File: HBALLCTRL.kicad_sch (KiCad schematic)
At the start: 9 parts

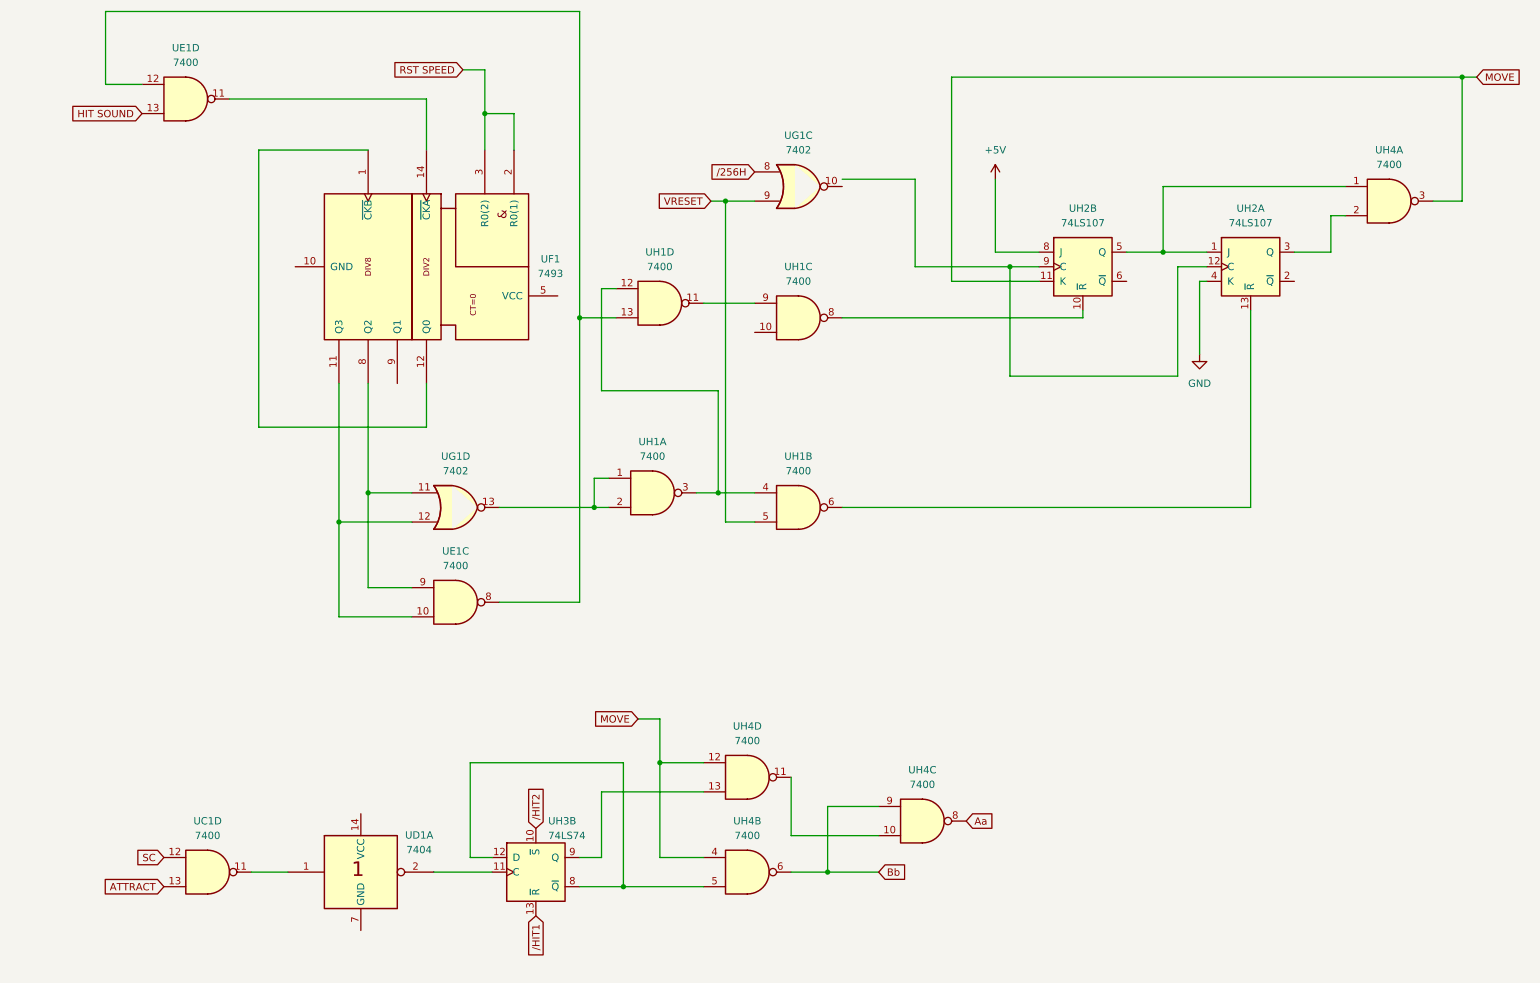
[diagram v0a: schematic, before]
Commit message: R20260915
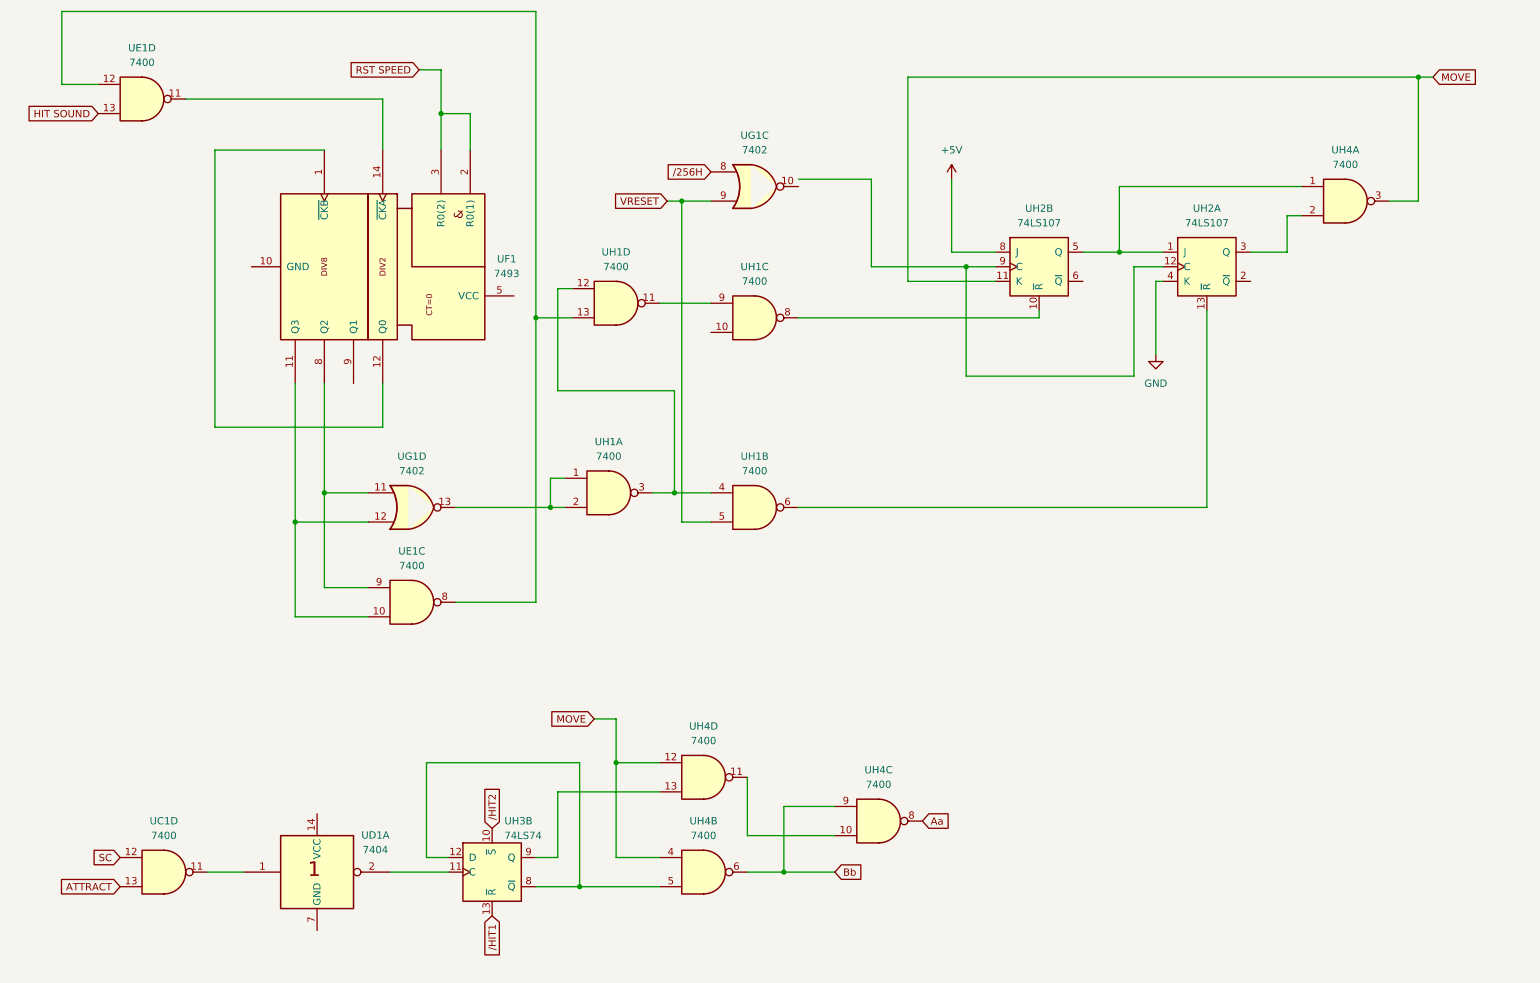
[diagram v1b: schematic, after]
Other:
- company: (none) -> Atari
- title: (none) -> PONG
- moved on the sheet: UC1D, UD1A, UE1C, UE1D, UF1, UG1C, UG1D, UH1A, UH1B, UH1C, UH1D, UH2A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
